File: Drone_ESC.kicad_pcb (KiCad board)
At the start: 6 copper layers, 60 x 37.5 mm, 62 parts, among them IC1 DRV8323RSRGZR, J1 Input, J2 62701021621, Q1 BSC014N06NS, Q2 BSC014N06NS, Q3 BSC014N06NS, Q4 BSC014N06NS, Q5 BSC014N06NS, Q6 BSC014N06NS, SW1 Reset, U1 STM32G473RCTx, Y1 XRCGB24M000F3A00R0

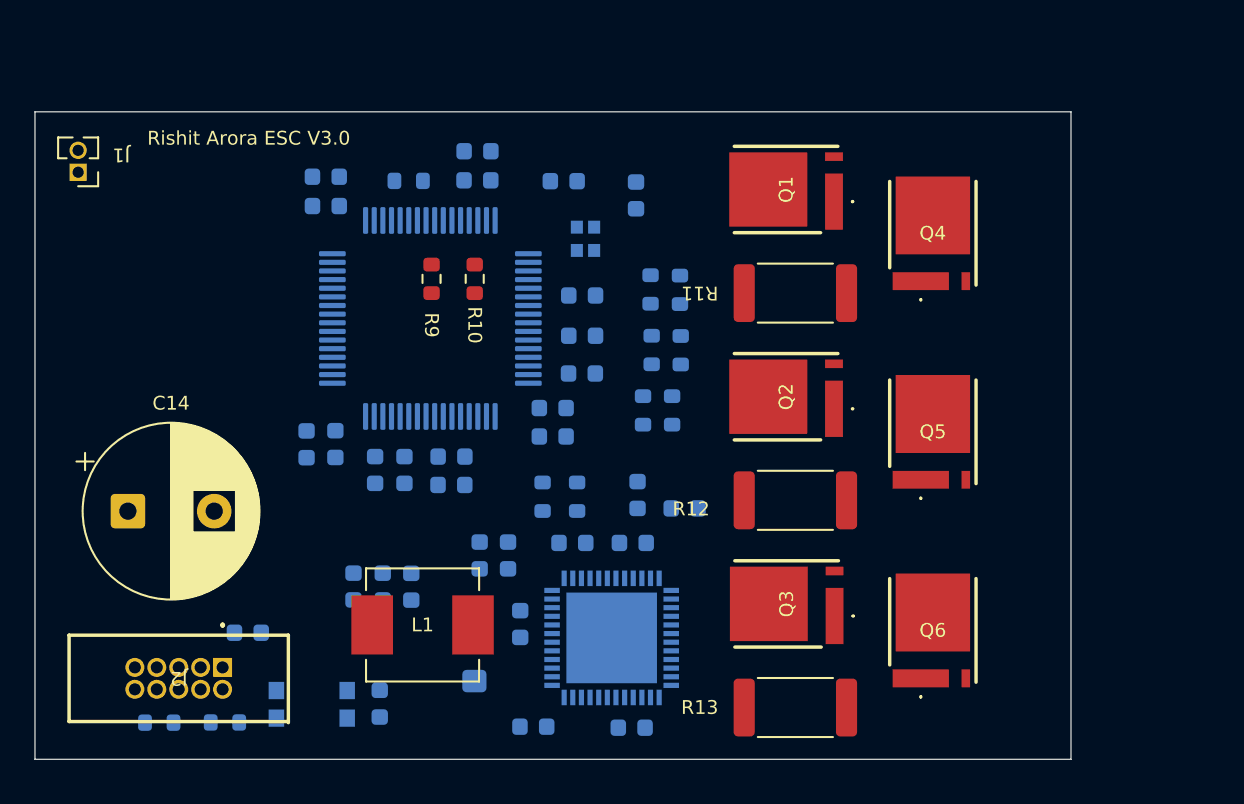
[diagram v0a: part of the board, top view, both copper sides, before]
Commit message: Almost done with routing
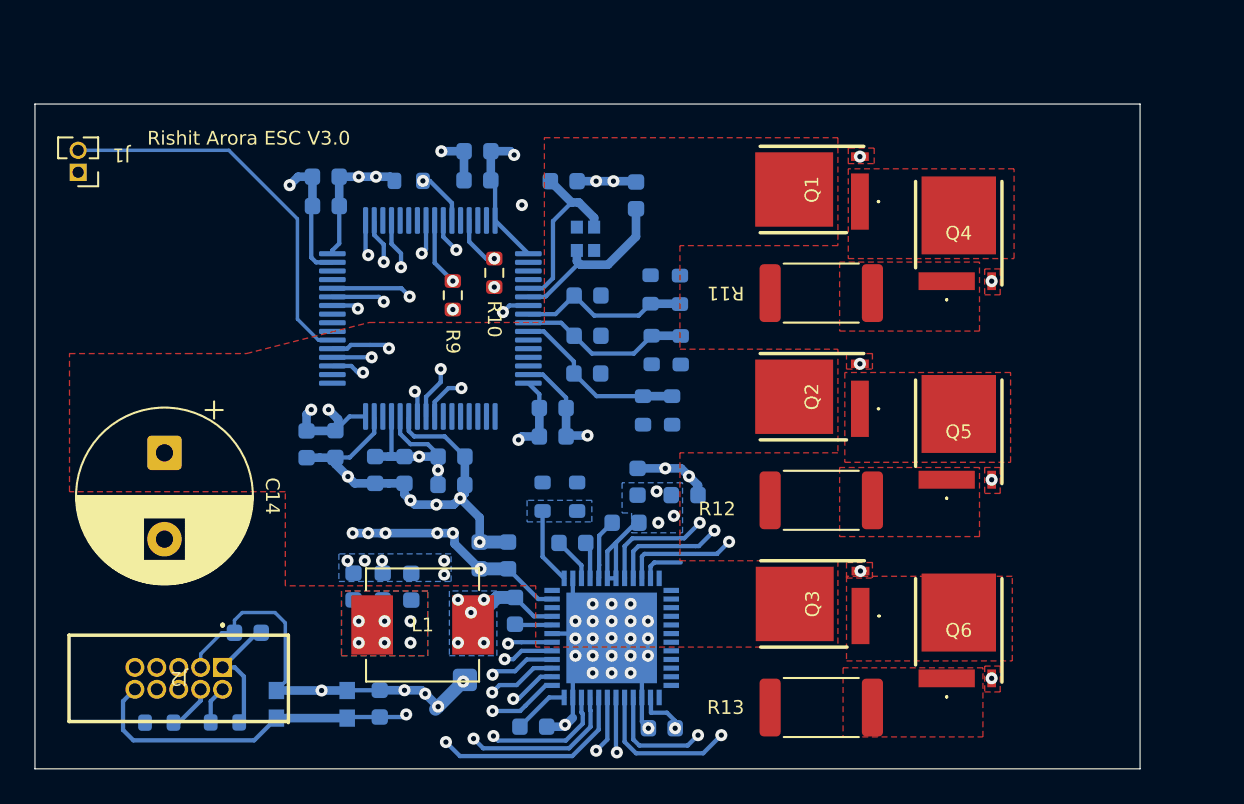
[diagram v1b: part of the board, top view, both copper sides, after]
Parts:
- moved C14 3.99 mm to (135.0, 106.2), turned to -90 degrees
- moved C22 1.74 mm to (163.8, 122.2)
- moved R9 1.56 mm to (151.7, 97.1)
- moved Q1 1.50 mm to (172.5, 91.0)
- moved Q2 1.50 mm to (172.5, 103.0)
- moved Q3 1.50 mm to (172.5, 115.0)
- moved Q4 1.50 mm to (181.0, 93.5)
- moved Q5 1.50 mm to (181.0, 105.0)
- moved Q6 1.50 mm to (181.0, 116.5)
- moved R11 1.50 mm to (173.0, 97.0)
- moved R12 1.50 mm to (173.0, 109.0)
- moved R13 1.50 mm to (173.0, 121.0)
- moved C28 1.24 mm to (161.7, 110.3)
- moved R10 1.19 mm to (154.1, 95.8)
- moved C24 0.82 mm to (155.3, 115.4)
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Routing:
- net RESET: track 0.00 -> 97.7 mm, vias 0 -> 2
- net GND: track 0.00 -> 96.2 mm, vias 0 -> 46
- net FAULT: track 0.00 -> 55.0 mm, vias 0 -> 3
- net +3.3V: track 0.00 -> 49.5 mm, vias 0 -> 16
- net SWO: track 0.00 -> 46.9 mm, vias 0 -> 1
- net SDO: track 0.00 -> 45.6 mm, vias 0 -> 2
- net DRIVER_EN: track 0.00 -> 43.0 mm, vias 0 -> 2
- net NSCS: track 0.00 -> 41.6 mm, vias 0 -> 2
- net SDI: track 0.00 -> 39.6 mm, vias 0 -> 2
- net SCLK: track 0.00 -> 39.0 mm, vias 0 -> 2
- net INHA: track 0.00 -> 37.9 mm, vias 0 -> 2
- net SWDCLK: track 0.00 -> 37.8 mm, vias 0 -> 1
- net INLA: track 0.00 -> 34.8 mm, vias 0 -> 2
- net INHC: track 0.00 -> 34.5 mm, vias 0 -> 2
- net INHB: track 0.00 -> 34.4 mm, vias 0 -> 2
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- added copper zone on B.Cu, net +3.3V
- added copper zone on F.Cu, net +3.3V
- added copper zone on In3.Cu, net +3.3V
- added copper zone on B.Cu, net +BATT
- added copper zone on F.Cu, net +BATT
- added copper zone on F.Cu, net GHA
- added copper zone on In2.Cu, net GHA
- added copper zone on F.Cu, net GHB
- added copper zone on In2.Cu, net GHB
- added copper zone on F.Cu, net GHC
- added copper zone on In2.Cu, net GHC
- added copper zone on F.Cu, net GLA
- added copper zone on In2.Cu, net GLA
- added copper zone on F.Cu, net GLB
- added copper zone on In2.Cu, net GLB
- added copper zone on F.Cu, net GLC
- added copper zone on In2.Cu, net GLC
- added copper zone on B.Cu, net GND
- added copper zone on In1.Cu, net GND
- added copper zone on B.Cu, net Net-(D1-K)
- added copper zone on B.Cu, net Net-(IC1-FB)
- added copper zone on F.Cu, net PHASE_A
- added copper zone on F.Cu, net PHASE_B
- added copper zone on F.Cu, net PHASE_C
- added copper zone on F.Cu, net SENSE_A
- added copper zone on F.Cu, net SENSE_B
- added copper zone on F.Cu, net SENSE_C
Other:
- board size 60 x 37.5 mm -> 64 x 38.5 mm
